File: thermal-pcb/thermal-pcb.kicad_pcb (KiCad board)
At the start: 2 copper layers, 98 x 56 mm, 60 parts, among them J2 Conn_01x14_Pin, J3 USB_C_Receptacle_USB2.0_16P, J4 Conn_01x04_Socket, J5 BATT_CONN, Q1 FS8205A, Q2 AO3415, U1 ESP32-S3-WROOM-1, U2 MCP73871, U3 MIC5504-3.3YM5, U4 DW01A, U5 MLX90640ESF-BAB-000-SP

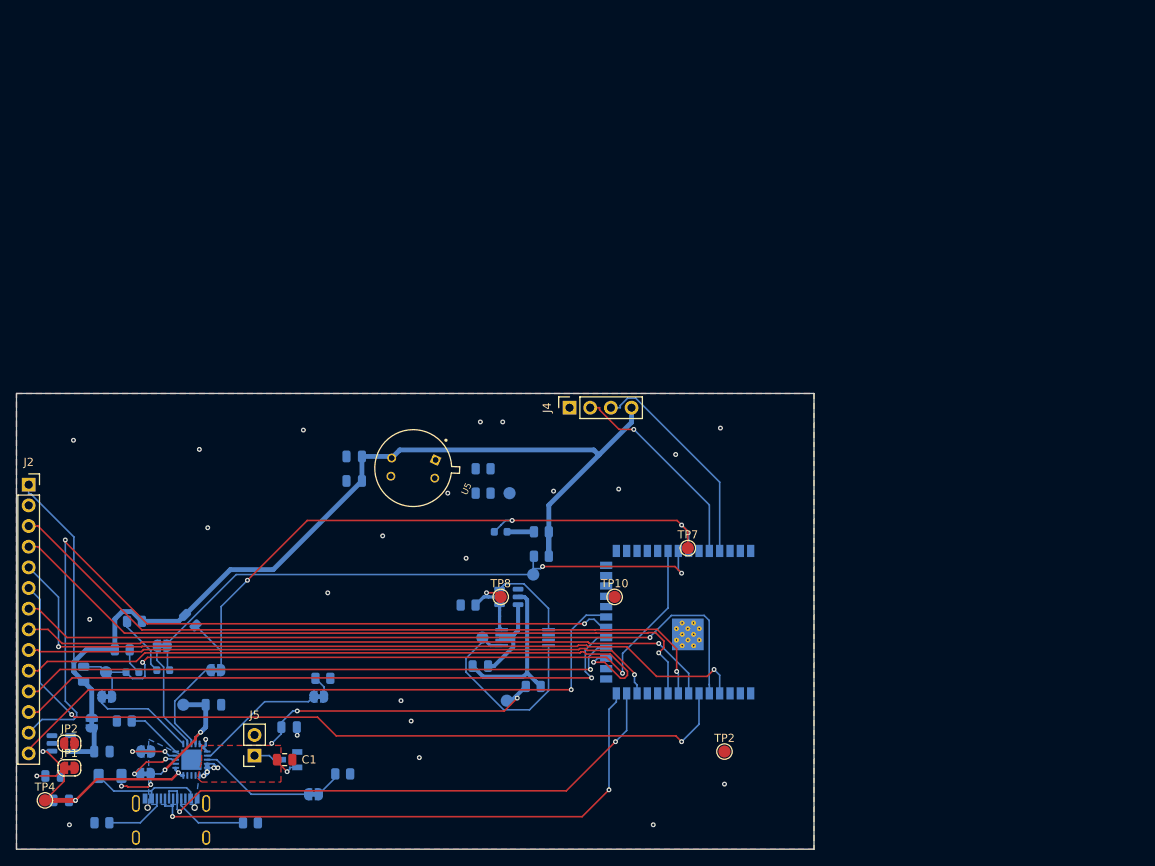
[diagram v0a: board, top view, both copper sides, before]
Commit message: work on pcb
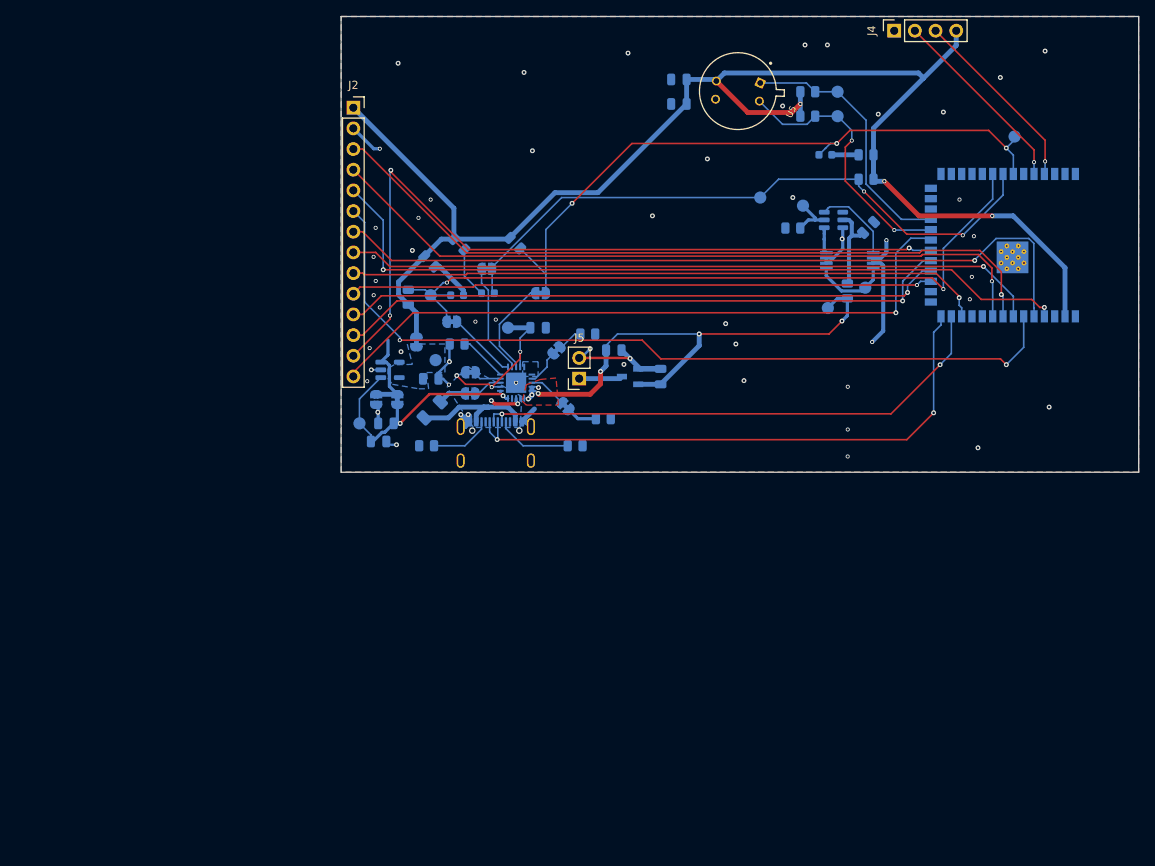
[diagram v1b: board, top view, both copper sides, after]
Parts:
- C1, JP1, JP2, TP10, TP2, TP4, TP7, TP8: moved to B.Cu
- J3: footprint Connector_USB:USB_C_Receptacle_G-Switch_GT-USB-7010ASV -> Connector_USB:USB_C_Receptacle_GCT_USB4105-xx-A_16P_TopMnt_Horizontal
- moved C6 72.0 mm to (158.2, 104.6), turned to 45 degrees
- moved TP10 67.9 mm to (154.4, 87.9)
- moved C1 66.0 mm to (132.6, 122.9), turned to 90 degrees
- moved TP7 64.6 mm to (176.1, 93.4)
- moved TP9 63.7 mm to (157.8, 112.0)
- moved Q2 63.0 mm to (128.9, 122.9)
- moved JP7 62.6 mm to (107.0, 116.2), turned to 180 degrees
- moved TP1 62.3 mm to (153.2, 114.5)
- moved R4 62.1 mm to (155.6, 112.4), turned to 90 degrees
- moved TH1 61.8 mm to (107.6, 118.9)
- moved JP10 61.5 mm to (102.6, 118.7)
- moved JP6 61.5 mm to (109.2, 125.0), turned to 180 degrees
- moved TP11 61.4 mm to (154.4, 90.9)
- moved JP4 61.3 mm to (109.3, 122.4), turned to 180 degrees
- moved U3 61.1 mm to (99.4, 122.1)
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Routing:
- net VCC: track 138.8 -> 181.1 mm, vias 0 -> 3
- net -BATT: track 18.5 -> 59.9 mm, vias 23 -> 54
- net I2C_SCL: track 0.00 -> 33.3 mm, vias 0 -> 2
- net I2C_SDA: track 0.00 -> 32.5 mm
- net +BATT: track 44.0 -> 64.2 mm, vias 8 -> 7
- net Net-(Q1-Pad1): track 26.3 -> 9.38 mm
- net Net-(JP5-A): track 16.1 -> 4.33 mm
- net LCD_T_CLK: track 82.9 -> 71.6 mm
- net Net-(JP1-B): track 0.00 -> 10.9 mm
- net Net-(U4-VCC): track 21.1 -> 10.5 mm
- net Net-(JP3-B): track 14.2 -> 4.67 mm
- net Net-(JP10-B): track 5.91 -> 0.00 mm
- net VBUS: track 22.8 -> 28.7 mm, vias 4 -> 5
- net LCD_T_DO: track 100.5 -> 95.4 mm, vias 2 -> 3
- net Net-(JP7-A): track 12.9 -> 8.55 mm
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- added copper zone on B.Cu, net Net-(JP10-B)
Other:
- board text added: "+BATT"
- board text added: "CS"
- board text added: "FUSE"
- board text added: "MSFP8"
- board text added: "PG"
- board text added: "PROG1"
- board text added: "PROG2"
- board text added: "PROG3"
- board text added: "SCL"
- board text added: "SDA"
- board text added: "STAT1"
- board text added: "STAT2"
- board text added: "VCC"
- board text added: "VIN"
- board text added: "VPCC"
